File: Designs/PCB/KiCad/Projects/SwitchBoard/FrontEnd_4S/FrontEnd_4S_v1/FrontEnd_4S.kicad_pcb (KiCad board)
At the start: 2 copper layers, 45 parts, among them J1 Conn_01x06_Female, J2 Header_Out_01x08, SW1 SW_Push, T1 Touch_Pad, T2 Touch_Pad, T3 Touch_Pad, T4 Touch_Pad, U1 APK2112.K-3.3, U2 STM32, U3 LoRa, U4 TTP223, U5 TTP223, U6 TTP223, U7 TTP223, Y1 32.768K, Y2 32Mhz

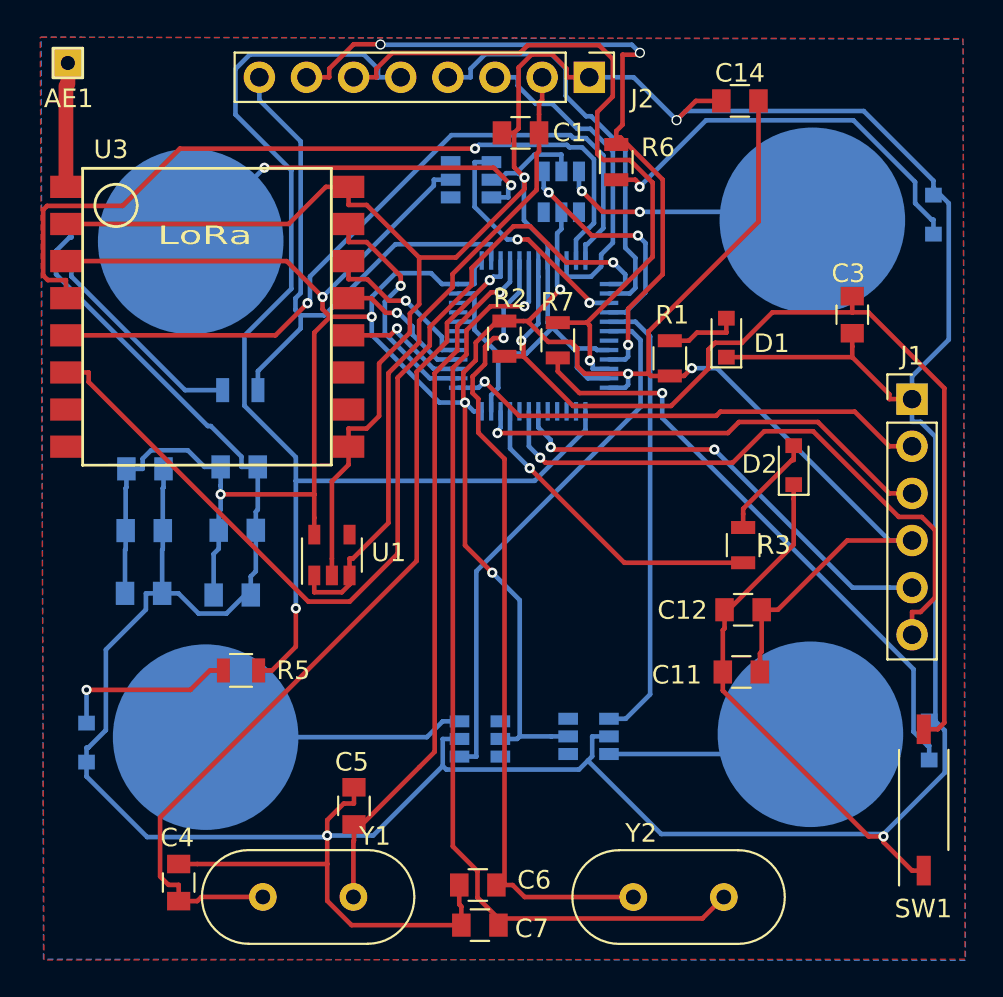
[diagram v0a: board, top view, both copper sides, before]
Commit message: learnings
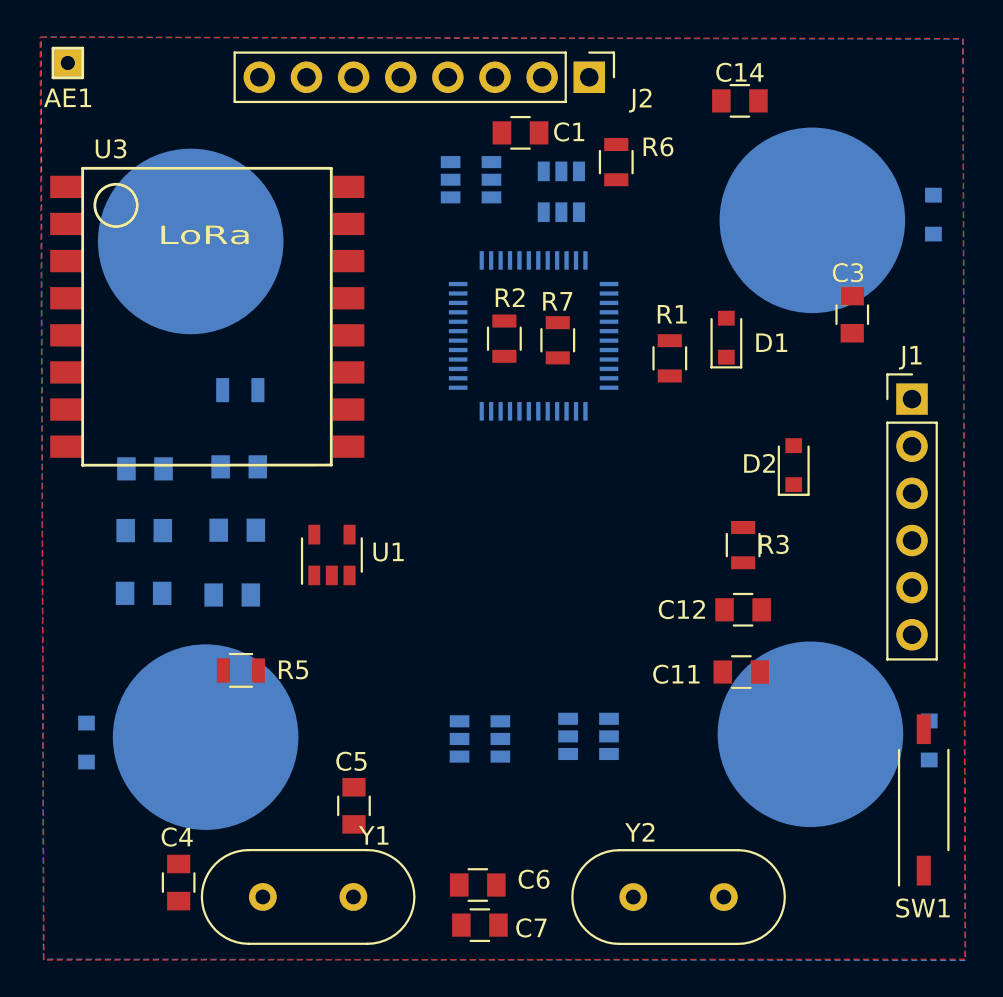
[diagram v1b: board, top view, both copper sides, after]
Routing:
- net /GND: track 326.5 -> 0.00 mm, vias 4 -> 0
- net /VCC3V3: track 177.3 -> 0.00 mm, vias 8 -> 0
- net /DSW_4: track 64.9 -> 0.00 mm, vias 1 -> 0
- net /RESET: track 55.0 -> 0.00 mm, vias 1 -> 0
- net /DIO1: track 53.1 -> 0.00 mm, vias 1 -> 0
- net /OSCOUT: track 52.2 -> 0.00 mm, vias 1 -> 0
- net /PC14: track 47.7 -> 0.00 mm, vias 1 -> 0
- net /OSCIN: track 43.4 -> 0.00 mm, vias 1 -> 0
- net /Reset_Lora: track 43.2 -> 0.00 mm, vias 1 -> 0
- net /DIO0: track 40.8 -> 0.00 mm, vias 1 -> 0
- net /DSW_2: track 40.0 -> 0.00 mm, vias 3 -> 0
- net /PC15: track 38.5 -> 0.00 mm, vias 1 -> 0
- net /DSW_3: track 38.4 -> 0.00 mm, vias 1 -> 0
- net /5V: track 34.7 -> 0.00 mm
- net /RX0: track 33.5 -> 0.00 mm, vias 1 -> 0
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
